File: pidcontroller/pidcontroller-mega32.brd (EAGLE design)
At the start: 100 x 75.4 mm, 19 parts, among them IC2 MAX3232CWE, IC3 MEGA32-A

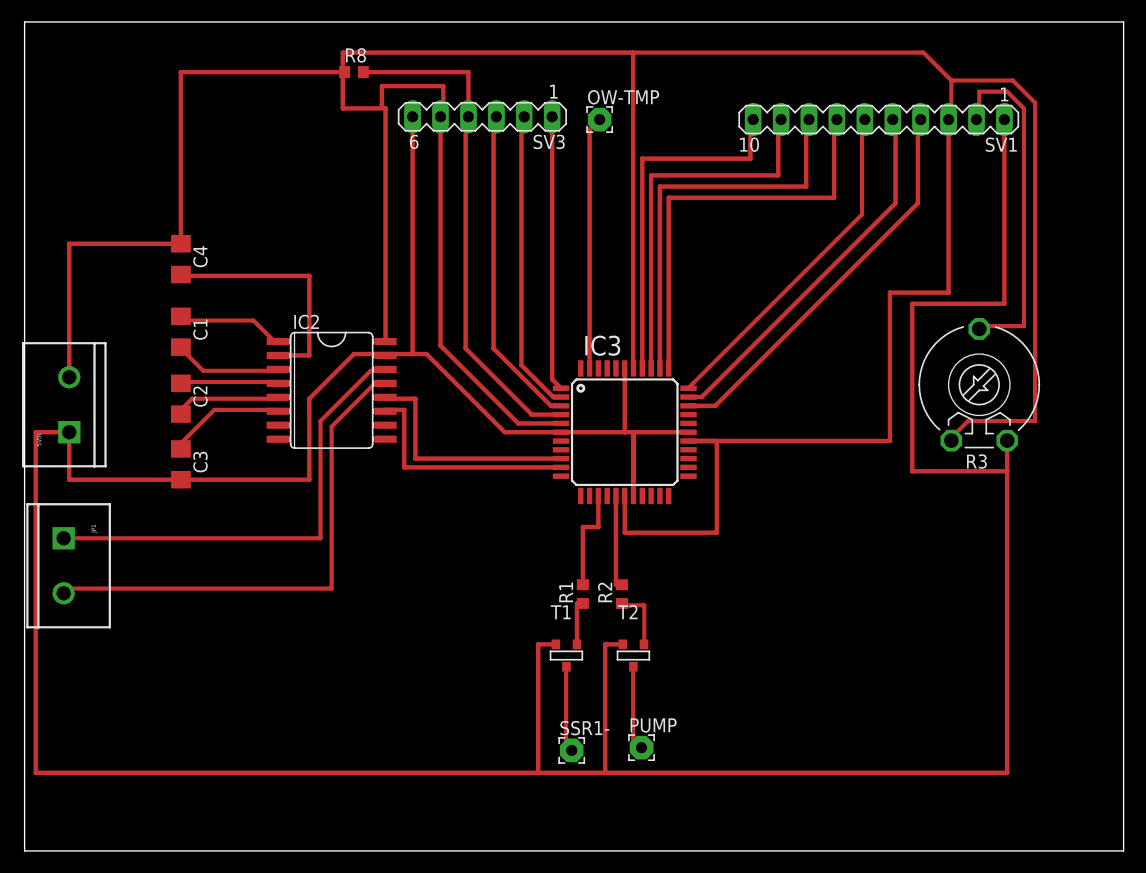
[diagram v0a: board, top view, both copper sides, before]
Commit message: cleanded up
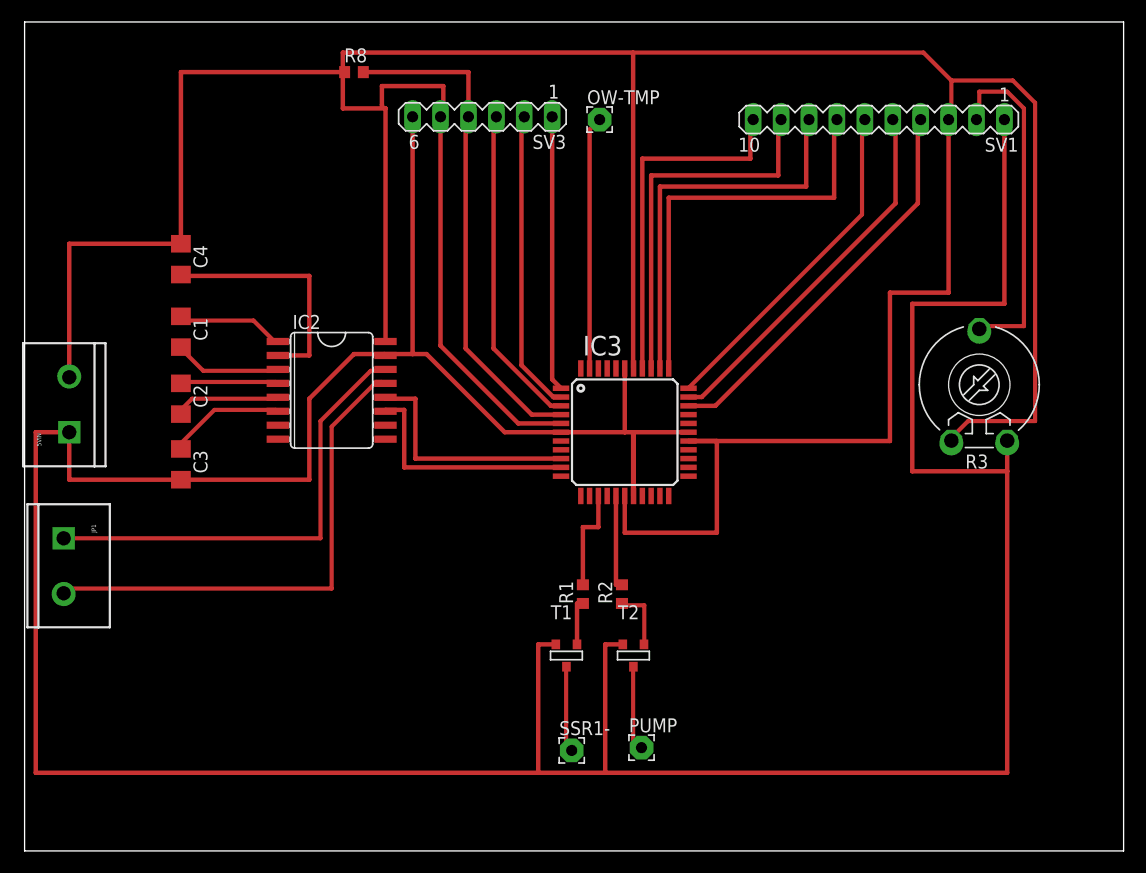
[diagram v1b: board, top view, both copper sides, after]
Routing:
- net VCC: vias 0 -> 1
- net GND: vias 0 -> 1
